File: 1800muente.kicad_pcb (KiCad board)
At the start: 2 copper layers, 371.5 x 104 mm, 170 parts, among them J1 Conn_01x04, K1 MX-1U, K10 MX-1U, K11 MX-1U, K12 MX-1U, K13 MX-1U, K14 MX-1U, K15 MX-1U, K16 MX-1U, K17 MX-1U, K18 MX-1U, K19 MX-1U, K2 MX-1U, K20 MX-1U, K21 MX-1U, K22 MX-1U, K23 MX-1U, K24 MX-1U, K25 MX-1U, K26 MX-1U, K27 MX-1U, K28 MX-1U, K29 MX-1U, K3 MX-1U, K30 MX-1U, K31 MX-1U, K32 MX-1U, K33 MX-1U, K34 MX-1U, K35 MX-1U, K36 MX-1U, K37 MX-1U, K38 MX-1U, K39 MX-1U, K4 MX-1U, K40 MX-1U, K41 MX-1U, K42 MX-1U, K43 MX-1U, K44 MX-1U, K45 MX-1U, K46 MX-1U, K47 MX-1U, K48 MX-1U, K49 MX-1U, K4_2 MX-1U, K5 MX-1U, K50 MX-1U, K51 MX-1U, K52 MX-1U, K53 MX-1U, K54 MX-1U, K55 MX-1U, K56 MX-1U, K57 MX-1U, K57_2 MX-1U, K58 MX-1U, K59 MX-1U, K6 MX-1U, K60 MX-1U, K61 MX-1U, K61_2 MX-1U, K62 MX-1U, K63 MX-1U, K64 MX-1U, K65 MX-1U, K66 MX-1U, K67 MX-1U, K68 MX-1U, K69 MX-1U, K7 MX-1U, K70 MX-1U, K71 MX-1U, K72 MX-1U, K73 MX-1U, K74 MX-1U, K75 MX-1U, K76 MX-1U, K77 MX-1U, K78 MX-1U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

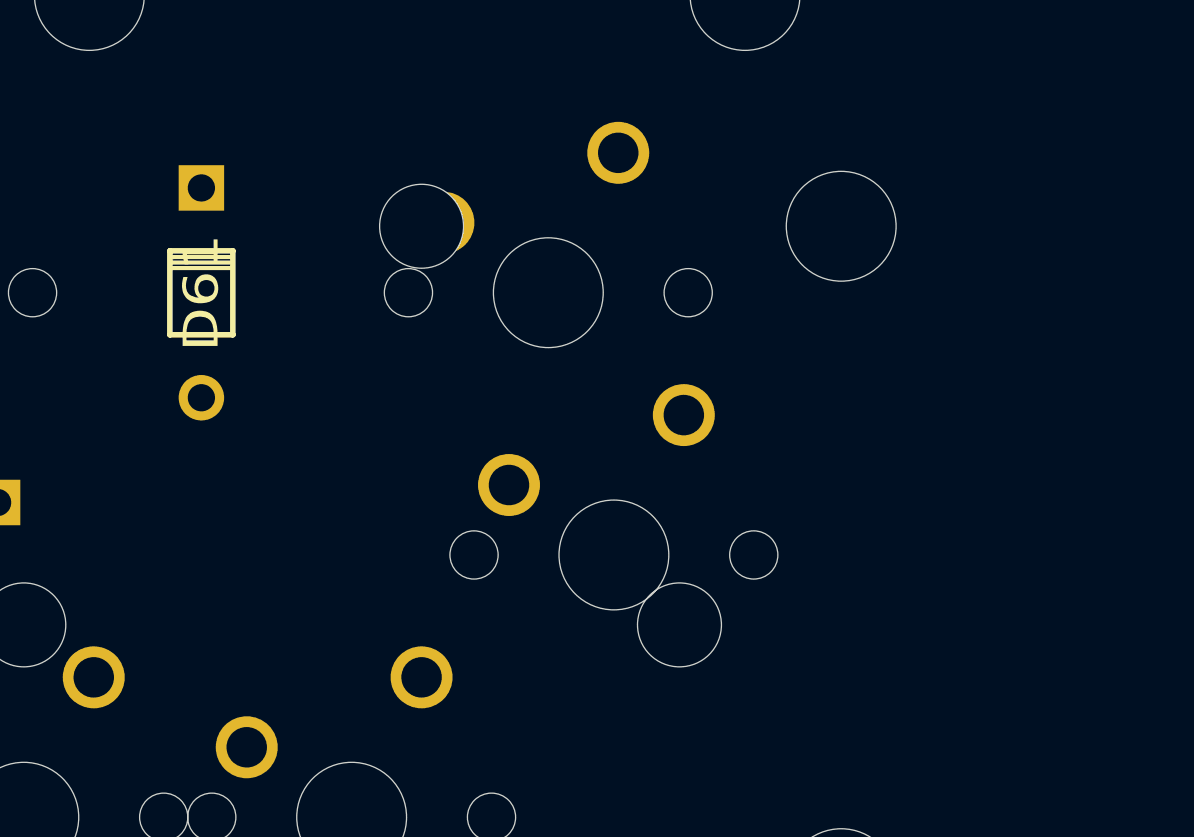
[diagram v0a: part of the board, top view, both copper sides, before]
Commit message: test
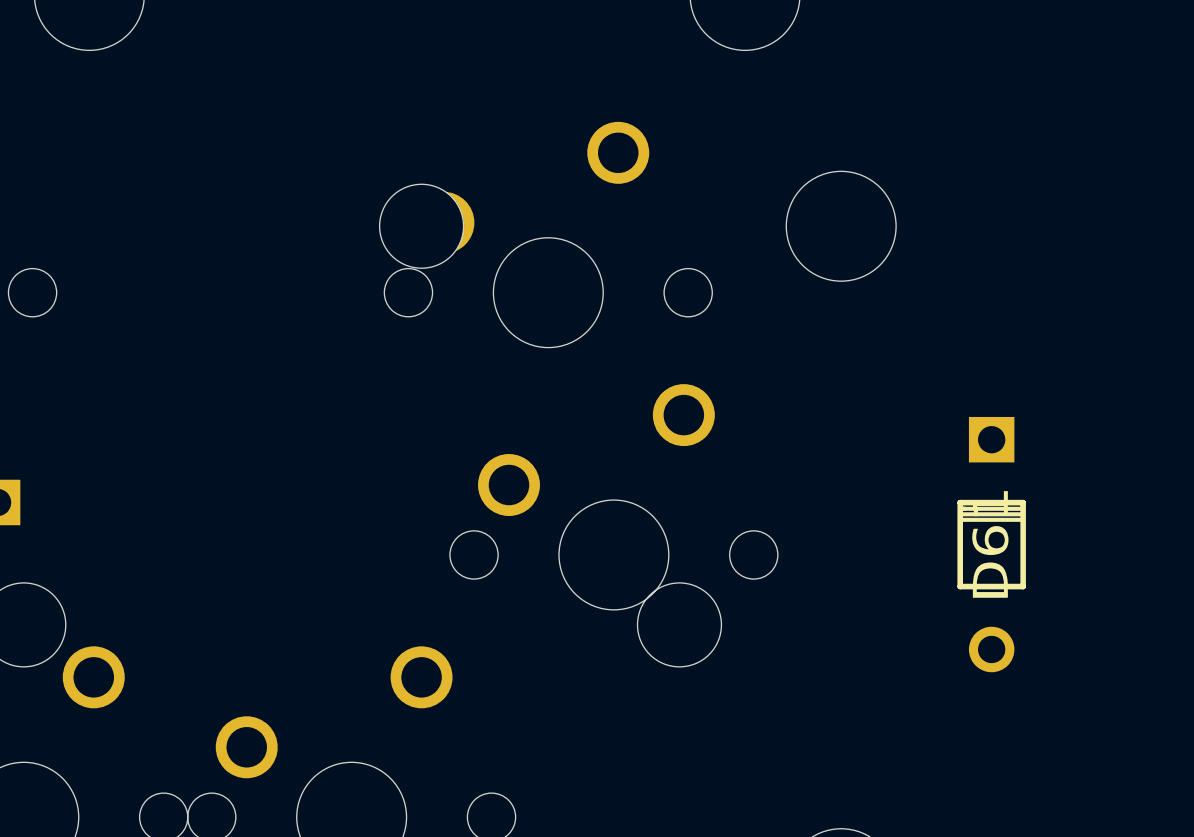
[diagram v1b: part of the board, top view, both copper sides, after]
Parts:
- moved D61 30.1 mm to (313.9, 129.8)
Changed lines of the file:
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@@
   )
   (module Keebio-Parts:Diode (layer F.Cu)
-    (at 285.242 120.65 90)
+    (at 313.944 129.794 90)
     (fp_text reference D61 (at 0 0 90) (layer F.SilkS)
       (effects (font (size 1.27 1.524) (thickness 0.2032)))
